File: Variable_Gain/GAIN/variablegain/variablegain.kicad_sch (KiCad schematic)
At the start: 7 parts, among them U1 OPA1641

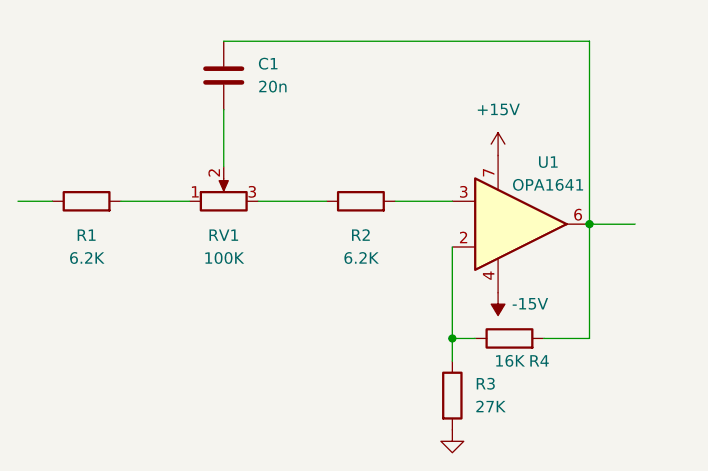
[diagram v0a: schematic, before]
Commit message: lpf, hpf, vg
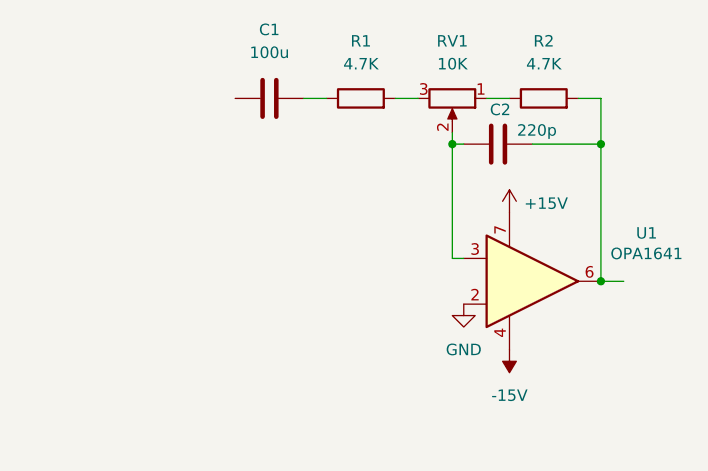
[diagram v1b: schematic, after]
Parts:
- removed R3: 27K, symbol Device:R
- removed R4: 16K, symbol Device:R
- added C2: 220p, symbol Device:C
- C1: value 20n -> 100u
- R1, R2: value 6.2K -> 4.7K
- RV1: value 100K -> 10K
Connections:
- net GND: now also U1.2 (-)
- net at U1.6: now also R2.2, C2.2; no longer C1.1
- net at RV1.2: now also U1.3 (+), C2.1; no longer C1.2
- net at R1.1: now also C1.1
- net at RV1.1: now also R2.1; no longer R1.2
- net at RV1.3: now also R1.2; no longer R2.1
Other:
- title: Variable LPF -> (none)

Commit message: started main schematic
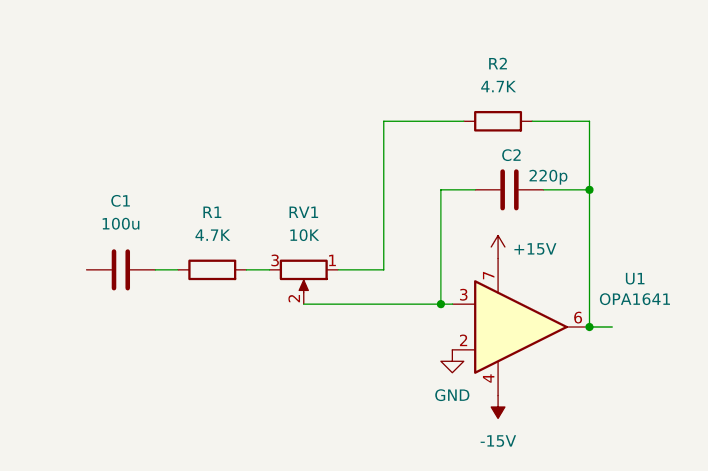
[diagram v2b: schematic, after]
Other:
- moved on the sheet: C1, C2, R1, R2, RV1, U1
